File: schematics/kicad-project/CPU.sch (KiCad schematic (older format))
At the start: 11 parts

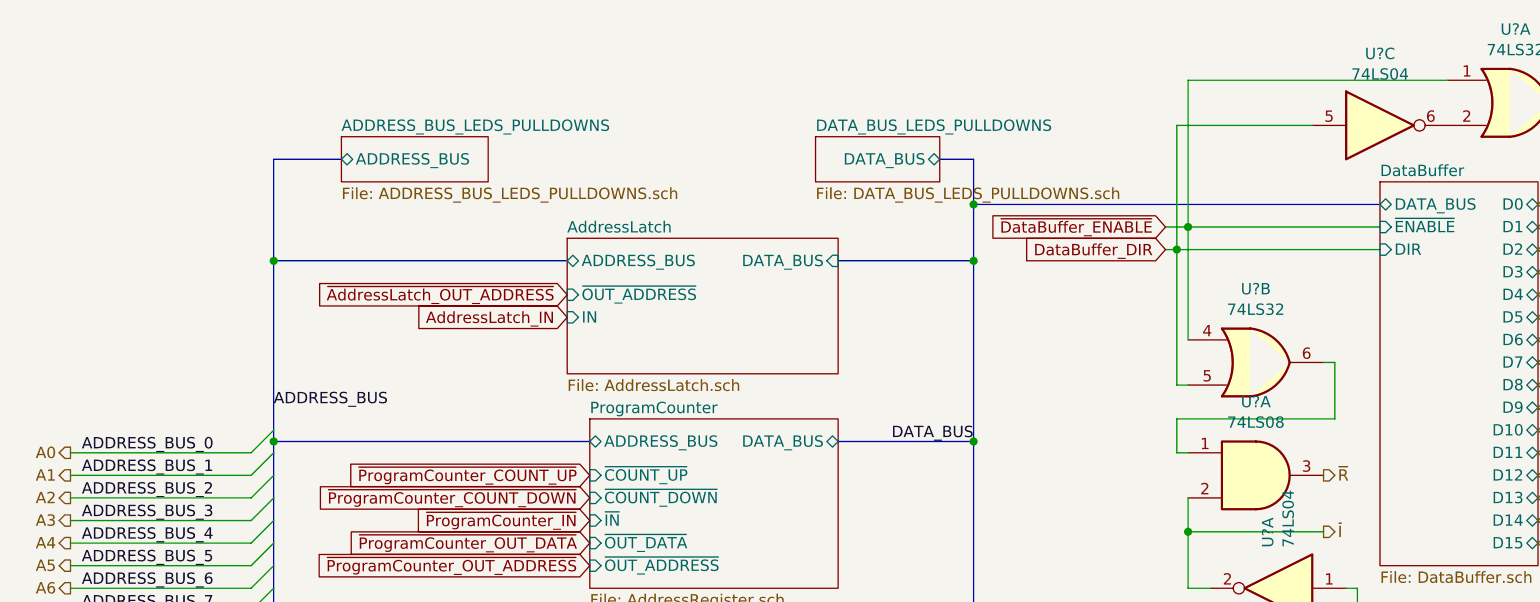
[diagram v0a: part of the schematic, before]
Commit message: Add base pointer register
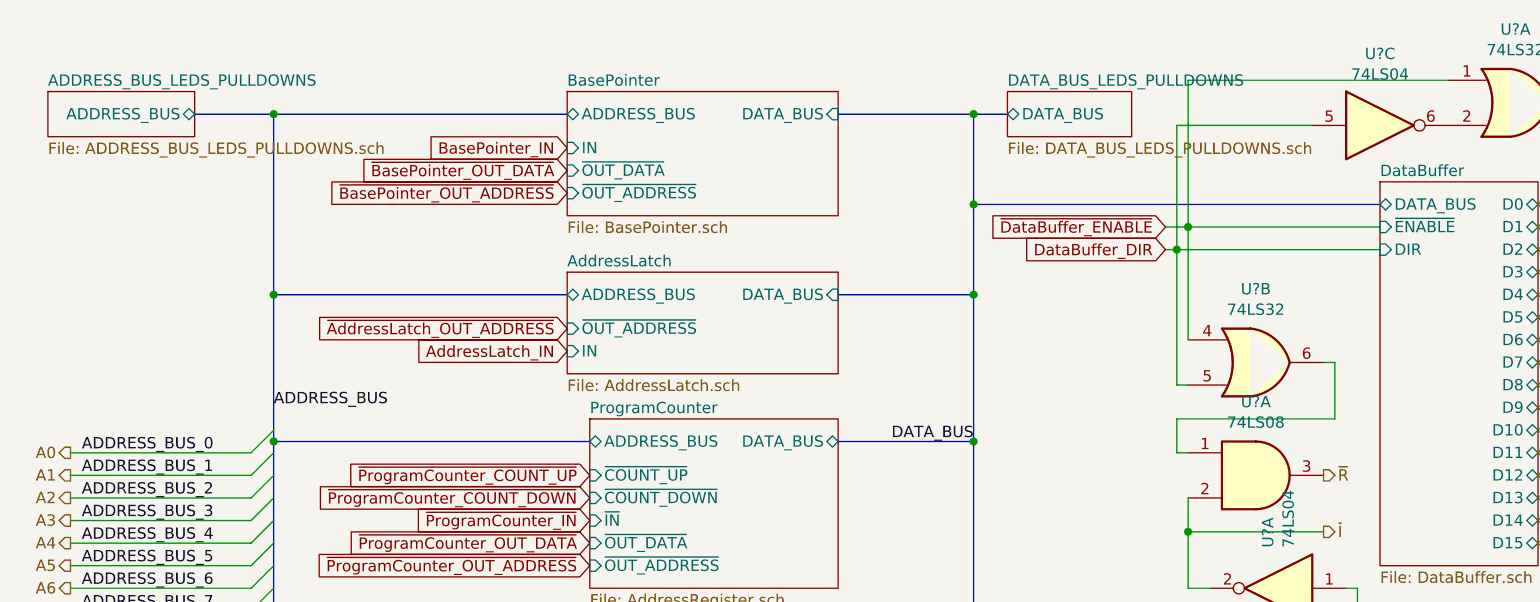
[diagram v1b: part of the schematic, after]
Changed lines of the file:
@@
 $Descr A4 8268 11693 portrait
 encoding utf-8
-Sheet 2 24
+Sheet 2 25
 Title ""
 Date ""
@@
 	4700 1300 6500 1300
 $Sheet
-S 2900 1450 1200 600
+S 2900 1600 1200 450
 U 5EB93191
 F0 "AddressLatch" 50
 F1 "AddressLatch.sch" 50
-F2 "DATA_BUS" I R 4100 1550 50
-F3 "IN" I L 2900 1800 50
-F4 "ADDRESS_BUS" T L 2900 1550 50
-F5 "~OUT_ADDRESS" I L 2900 1700 50
-$EndSheet
-Text GLabel 2900 1700 0    50   Input ~ 0
+F2 "DATA_BUS" I R 4100 1700 50
+F3 "IN" I L 2900 1950 50
+F4 "ADDRESS_BUS" T L 2900 1700 50
+F5 "~OUT_ADDRESS" I L 2900 1850 50
+$EndSheet
+Text GLabel 2900 1850 0    50   Input ~ 0
 ~AddressLatch_OUT_ADDRESS
-Text GLabel 2900 1800 0    50   Input ~ 0
+Text GLabel 2900 1950 0    50   Input ~ 0
 AddressLatch_IN
 Wire Bus Line
-	2900 1550 1600 1550
-Wire Bus Line
-	4100 1550 4700 1550
+	2900 1700 1600 1700
+Wire Bus Line
+	4100 1700 4700 1700
 Text HLabel 7400 850  2    50   Output ~ 0
 ~W
@@
 $EndSheet
 $Sheet
-S 4000 1000 550  200
+S 4850 800  550  200
 U 60996BF7
 F0 "DATA_BUS_LEDS_PULLDOWNS" 50
 F1 "DATA_BUS_LEDS_PULLDOWNS.sch" 50
-F2 "DATA_BUS" T R 4550 1100 50
-$EndSheet
-$Sheet
-S 1900 1000 650  200
-U 60A197D9
-F0 "ADDRESS_BUS_LEDS_PULLDOWNS" 50
-F1 "ADDRESS_BUS_LEDS_PULLDOWNS.sch" 50
-F2 "ADDRESS_BUS" T L 1900 1100 50
-$EndSheet
-Wire Bus Line
-	1600 1550 1600 1100
-Connection ~ 1600 1550
-Wire Bus Line
-	1600 1100 1900 1100
-Wire Bus Line
-	4700 1100 4700 1300
-Connection ~ 4700 1550
+F2 "DATA_BUS" T L 4850 900 50
+$EndSheet
 $Sheet
 S 3000 2250 1100 750
@@
 Text HLabel 7450 4750 2    50   3State ~ 0
 D15
-Wire Bus Line
-	4550 1100 4700 1100
 Connection ~ 4700 4100
 Wire Bus Line
@@
 	4700 3400 4700 4100
 Connection ~ 4700 1300
-Wire Bus Line
-	4700 1300 4700 1550
-Wire Bus Line
-	4700 1550 4700 2350
 $Comp
 L 74xx:74LS04 U?
@@
 Wire Wire Line
 	5600 1500 6500 1500
-Wire Bus Line
-	1600 1550 1600 2350
+$Sheet
+S 600  800  650  200
+U 60A197D9
+F0 "ADDRESS_BUS_LEDS_PULLDOWNS" 50
+F1 "ADDRESS_BUS_LEDS_PULLDOWNS.sch" 50
+F2 "ADDRESS_BUS" T R 1250 900 50
+$EndSheet
+Wire Bus Line
+	4850 900  4700 900
+Wire Bus Line
+	1250 900  1600 900
+Connection ~ 1600 1700
+Connection ~ 4700 1700
+Wire Bus Line
+	4700 1700 4700 2350
+Wire Bus Line
+	4700 1300 4700 1700
+$Sheet
+S 2900 800  1200 550
+U 6132941C
+F0 "BasePointer" 50
+F1 "BasePointer.sch" 50
+F2 "DATA_BUS" I R 4100 900 50
+F3 "~OUT_DATA" I L 2900 1150 50
+F4 "IN" I L 2900 1050 50
+F5 "~OUT_ADDRESS" I L 2900 1250 50
+F6 "ADDRESS_BUS" T L 2900 900 50
+$EndSheet
+Wire Bus Line
+	2900 900  1600 900
+Wire Bus Line
+	4100 900  4700 900
+Text GLabel 2900 1050 0    50   Input ~ 0
+BasePointer_IN
+Text GLabel 2900 1150 0    50   Input ~ 0
+~BasePointer_OUT_DATA
+Text GLabel 2900 1250 0    50   Input ~ 0
+~BasePointer_OUT_ADDRESS
+Connection ~ 1600 900
+Wire Bus Line
+	1600 900  1600 1700
+Connection ~ 4700 900
+Wire Bus Line
+	4700 900  4700 1300
+Wire Bus Line
+	1600 1700 1600 2350
 Wire Bus Line
 	1600 3400 1600 4450
